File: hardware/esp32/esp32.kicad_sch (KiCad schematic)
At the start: 21 parts, among them J1 Conn_01x02, J2 Conn_01x02, J3 Conn_01x02, J4 Conn_01x02, J5 Conn_01x02, J6 Conn_01x02, SW1 RESET, SW2 BOOT, U1 USBLC6-2SC6, U2 ESP32-S3-MINI-1-N8

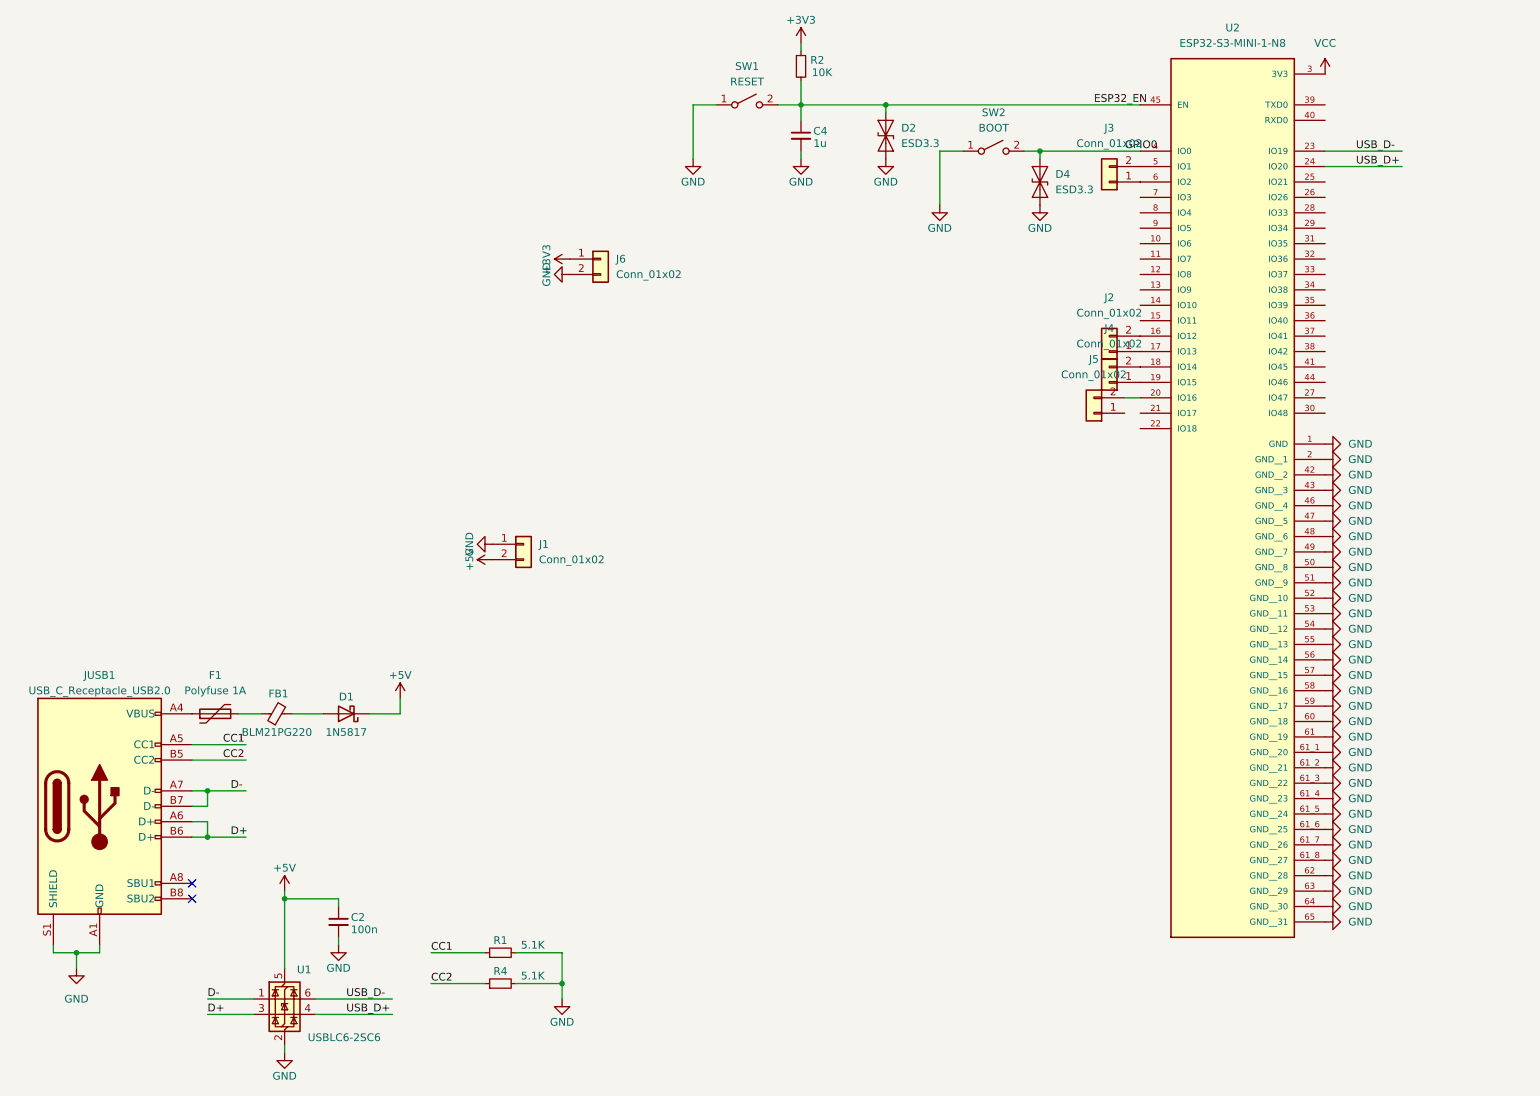
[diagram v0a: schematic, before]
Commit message: esp32
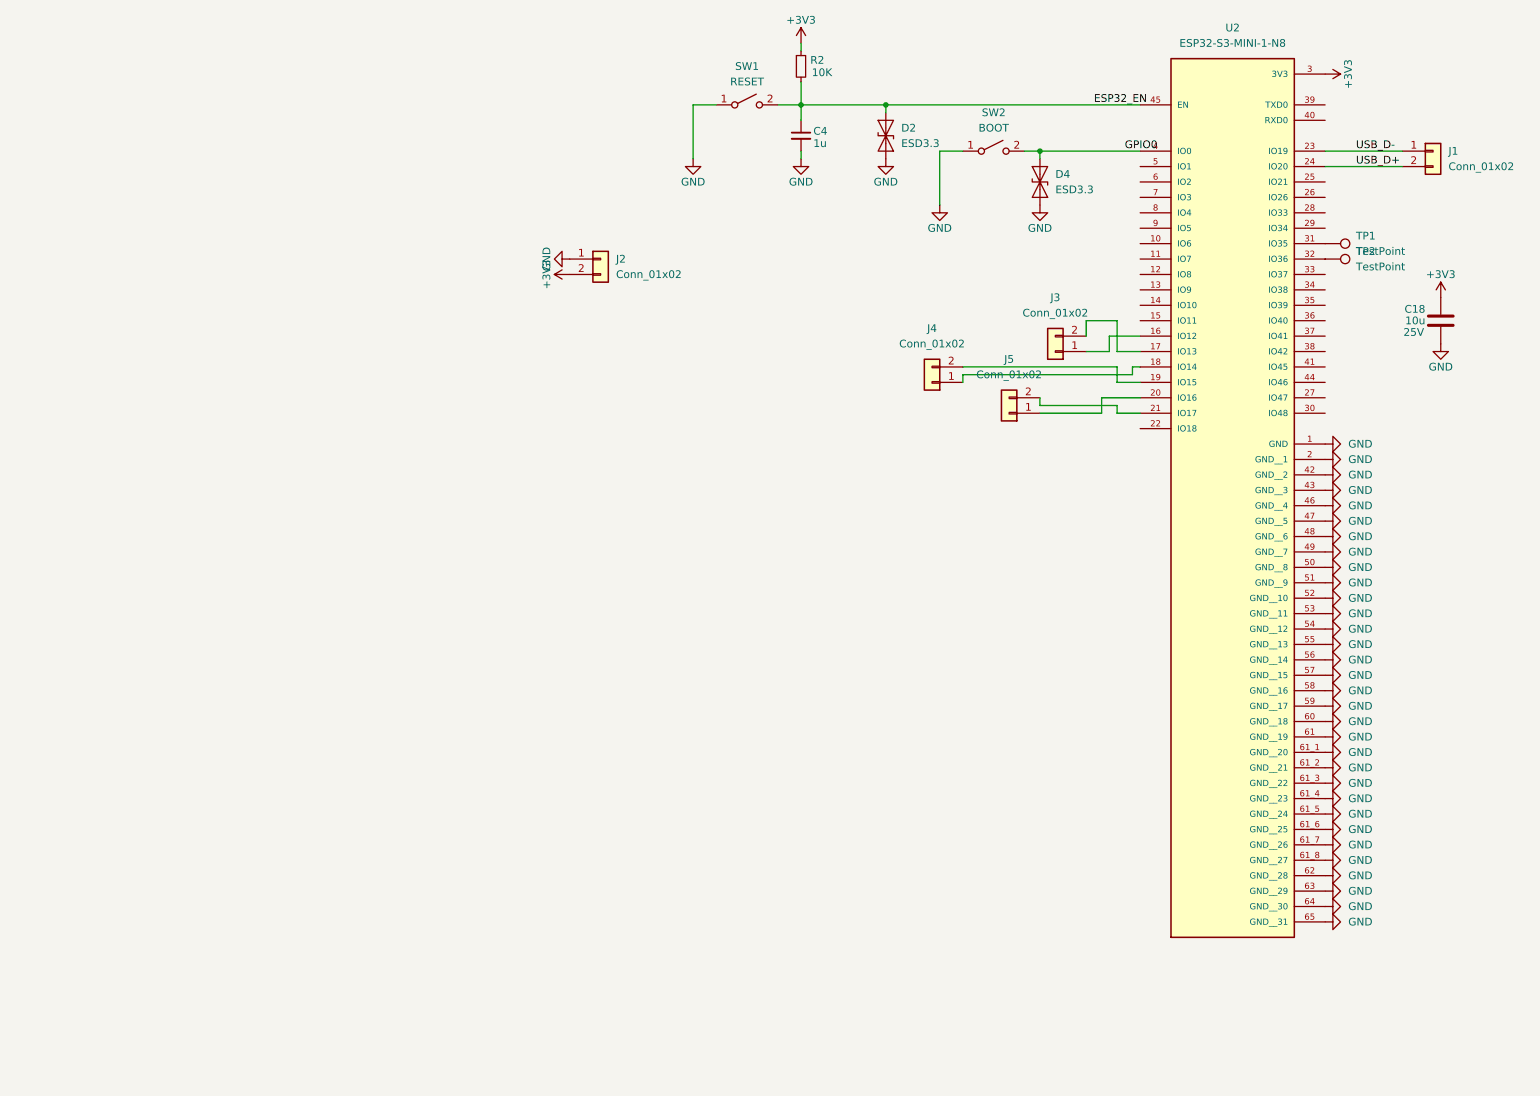
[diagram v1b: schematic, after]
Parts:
- removed C2: 100n, Capacitor_SMD:C_0402_1005Metric_Pad0.74x0.62mm_HandSolder, symbol Morten_Library.kicad_sym_9:C_Small
- removed D1: 1N5817, Diode_SMD:D_SOD-123, symbol Morten_Library.kicad_sym_9:1N5817
- removed F1: Polyfuse 1A, Fuse:Fuse_1206_3216Metric, symbol Morten_Library.kicad_sym_9:Polyfuse
- removed FB1: BLM21PG220, Inductor_SMD:L_0805_2012Metric, symbol Morten_Library.kicad_sym_9:FerriteBead_Small
- removed J6: Conn_01x02, Connector_JST:JST_SHL_SM02B-SHLS-TF_1x02-1MP_P1.00mm_Horizontal, symbol Connector_Generic:Conn_01x02
- removed JUSB1: USB_C_Receptacle_USB2.0, Connector_USB:USB_C_Receptacle_GCT_USB4105-xx-A_16P_TopMnt_Horizontal, symbol Connector:USB_C_Receptacle_USB2.0
- removed R1, R4: 5.1K, Resistor_SMD:R_0402_1005Metric, symbol Morten_Library.kicad_sym_9:R_Small
- removed U1: USBLC6-2SC6, Package_TO_SOT_SMD:SOT-23-6, symbol Morten_Library.kicad_sym_9:USBLC6-2SC6_1
- added C18: 10u, Capacitor_SMD:C_0603_1608Metric, symbol Device:C
- added TP1, TP2: TestPoint, TestPoint:TestPoint_Pad_1.0x1.0mm, symbol Connector:TestPoint
- J2: footprint Connector_JST:JST_SHL_SM02B-SHLS-TF_1x02-1MP_P1.00mm_Horizontal -> Connector_JST:JST_ZH_S2B-ZR-SM4A-TF_1x02-1MP_P1.50mm_Horizontal; LCSC C160402 -> C157930
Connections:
- net +5V is gone; now on net USB_D+: J1.2 (Pin_2)
- net VCC is gone; now on net +3V3: U2.3 (3V3)
- net +3V3: now also J2.2 (Pin_2), C18.1
- net GND: now also J2.1 (Pin_1), C18.2; no longer J1.1 (Pin_1)
- net USB_D-: now also J1.1 (Pin_1)
- net at U2.16 (IO12): now also J3.1 (Pin_1); no longer J2.2 (Pin_2)
- net at U2.17 (IO13): now also J3.2 (Pin_2); no longer J2.1 (Pin_1)
- net at U2.18 (IO14): now also J4.1 (Pin_1); no longer J4.2 (Pin_2)
- net at U2.19 (IO15): now also J4.2 (Pin_2); no longer J4.1 (Pin_1)
- net at U2.20 (IO16): now also J5.1 (Pin_1); no longer J5.2 (Pin_2)
- net at U2.21 (IO17): now also J5.2 (Pin_2)
- net at U2.31 (IO35): now also TP1.1
- net at U2.32 (IO36): now also TP2.1
- net at U2.5 (IO1): no longer J3.2 (Pin_2)
- net at U2.6 (IO2): no longer J3.1 (Pin_1)
- no-connect marks 2 -> 0
